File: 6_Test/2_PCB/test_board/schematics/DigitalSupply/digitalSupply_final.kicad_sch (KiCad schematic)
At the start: 10 parts, among them U4 LDO_Digital_Supply

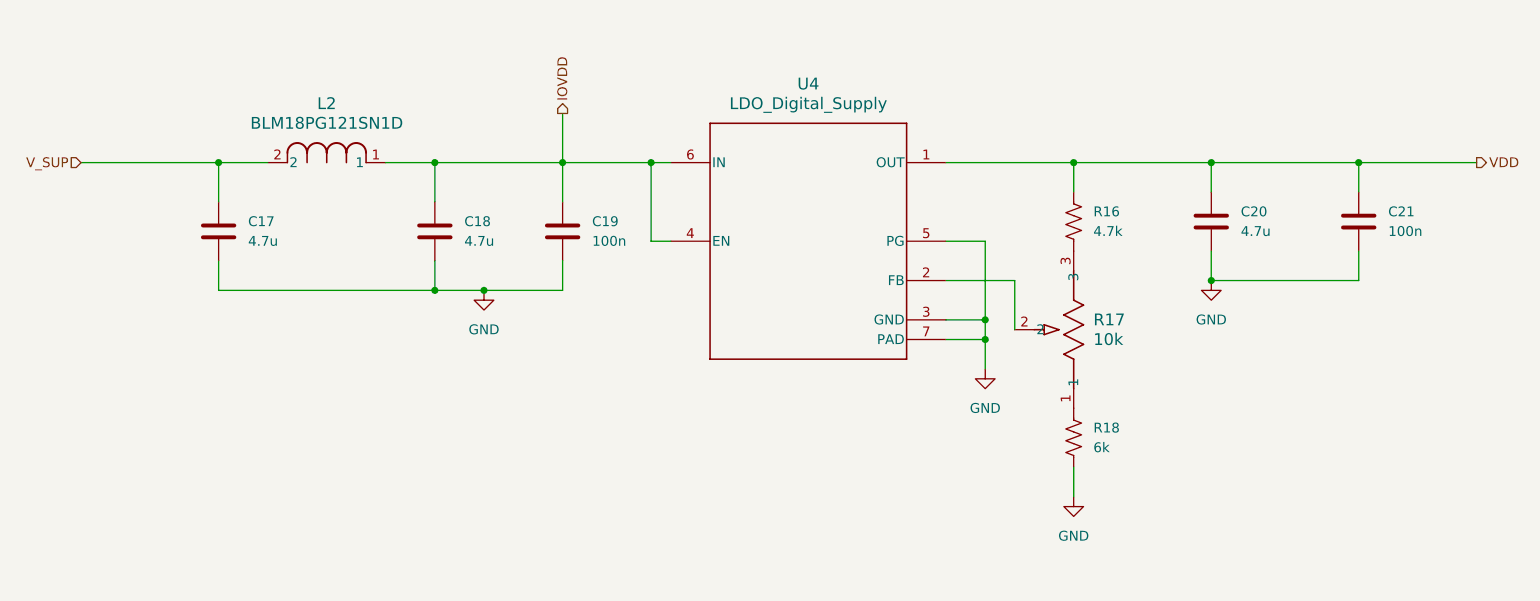
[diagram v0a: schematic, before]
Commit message: Adjusted Edits 11_25_24
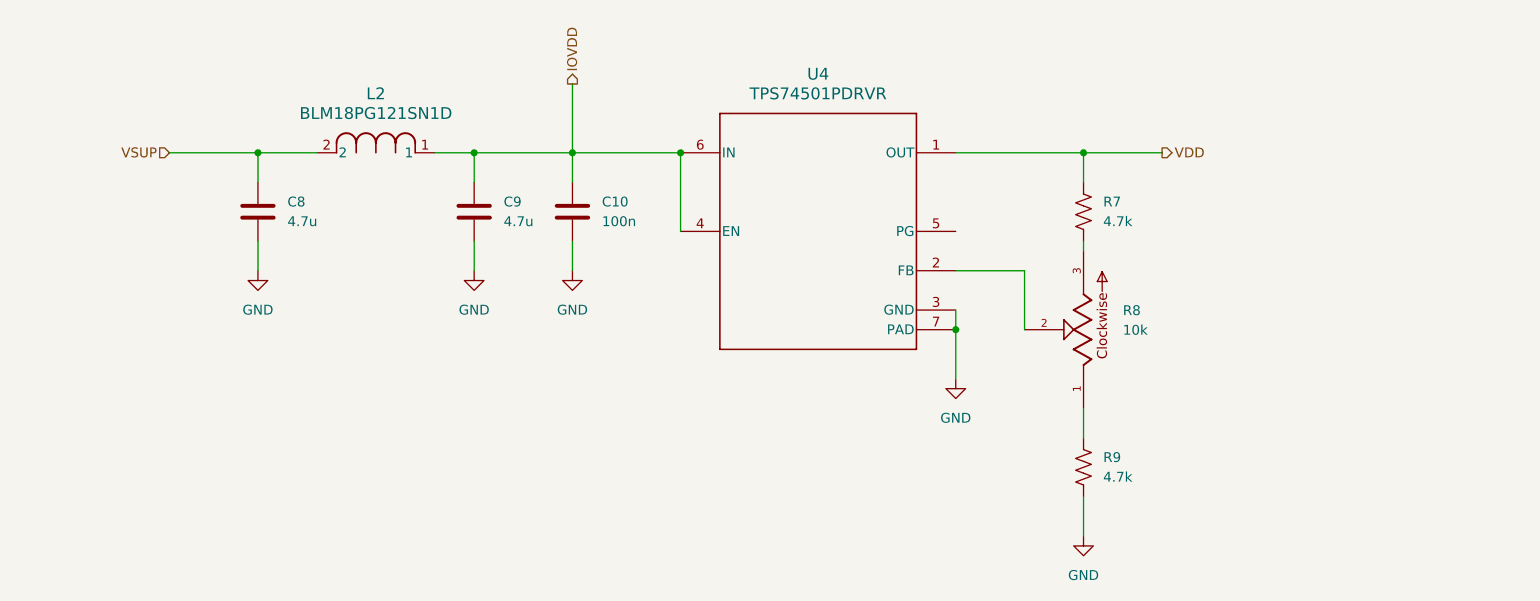
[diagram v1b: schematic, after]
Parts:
- removed C17, C18, C20: 4.7u, Capacitor_SMD:C_0201_0603Metric, symbol Device:C
- removed C19, C21: 100n, Capacitor_SMD:C_0201_0603Metric, symbol Device:C
- removed L2: BLM18PG121SN1D, ferriteBead120OhmFootprints:IND_BLM18_0603_MUR, symbol ferritebead:BLM18PG121SN1D
- removed R16: 4.7k, Resistor_SMD:R_0201_0603Metric, symbol Device:R_US
- removed R17: 10k, potentiometer_10turn:potentiometer_10turn, symbol pot10turn:PV37W103C01B00
- removed R18: 6k, Resistor_SMD:R_0201_0603Metric, symbol Device:R_US
- removed U4: LDO_Digital_Supply, tps745Footprints:DRV0006A_NV, symbol tps745:TPS74501PDRVR
- added C10: 100n, Capacitor_SMD:C_0402_1005Metric, symbol Device:C
- added C8, C9: 4.7u, Capacitor_SMD:C_0603_1608Metric, symbol Device:C
- added L2: BLM18PG121SN1D, ferriteBead120OhmFootprints:IND_BLM18_0603_MUR, symbol 2024-09-16_06-39-17:BLM18PG121SN1D
- added R7, R9: 4.7k, symbol Device:R_US
- added R8: 10k, ECE628_lib:potentiometer_10turn, symbol pot_10turn:PV37W103C01B00
- added U4: TPS74501PDRVR, tps745Footprints:DRV0006A, symbol TPS745_LDO:TPS74501PDRVR
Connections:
- net GND: now also C10.2, C8.2, C9.2, R9.2, U4.3 (GND), U4.7 (PAD)
- net IOVDD: now also C10.1, C9.1, L2.1, U4.4 (EN), U4.6 (IN)
- net VDD: now also R7.1, U4.1 (OUT)
- new net: R8.1, R9.1
- new net: R8.2, U4.2 (FB)
- new net: R7.2, R8.3
- new net VSUP: C8.1, L2.2
